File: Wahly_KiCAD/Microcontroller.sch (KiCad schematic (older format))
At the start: 21 parts, among them SW1 SW_SPDT, U5 STM32F302C8Tx, U6 W25Q32JVSS, Y1 16MHz

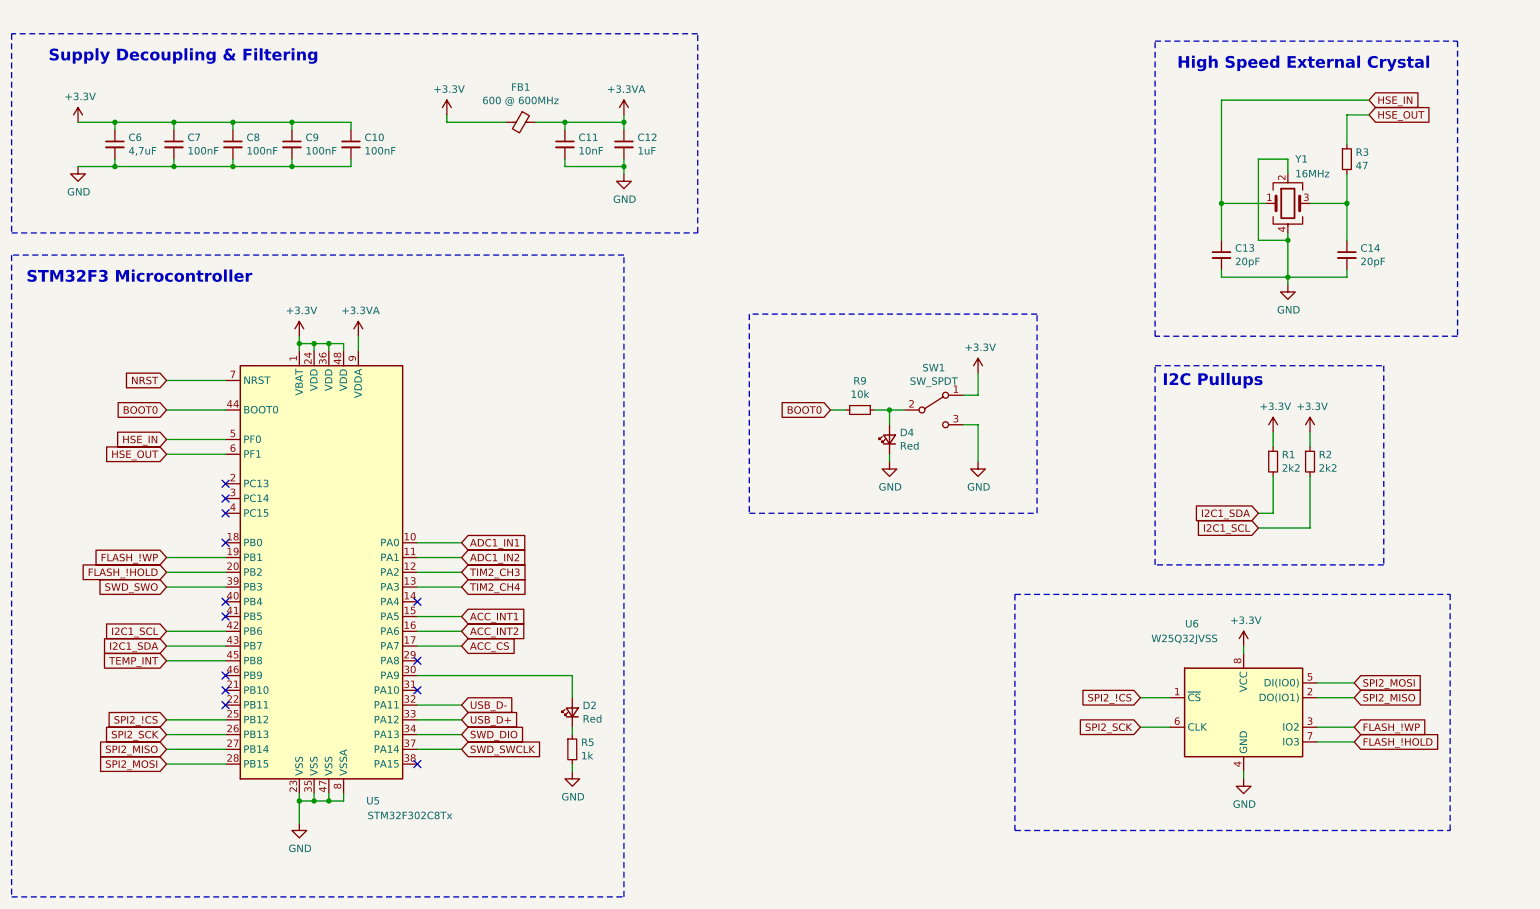
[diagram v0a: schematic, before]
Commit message: pdf schematic
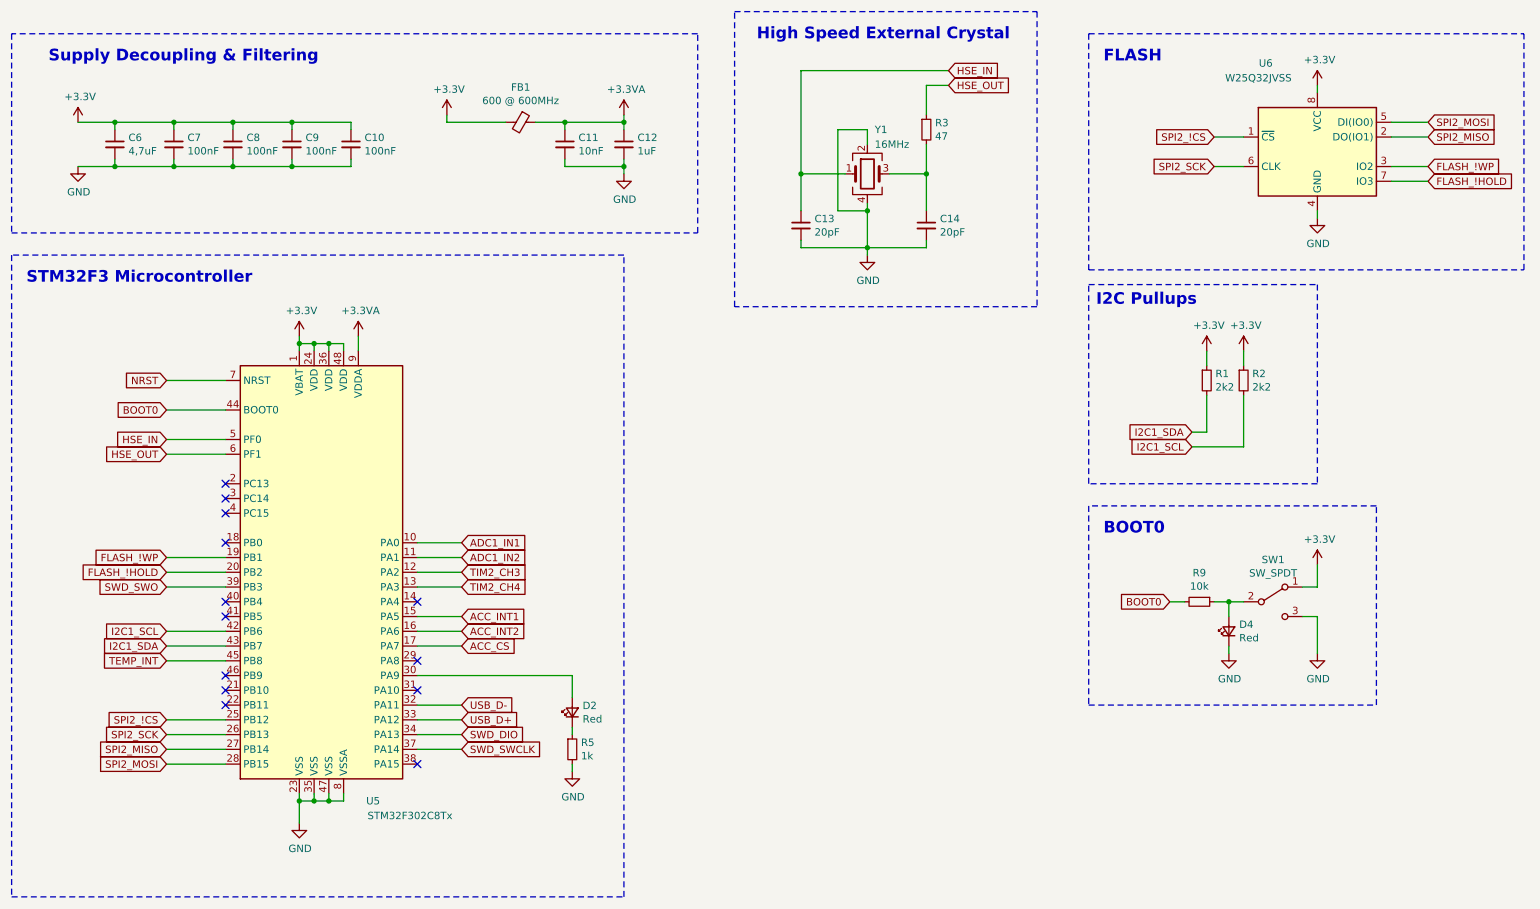
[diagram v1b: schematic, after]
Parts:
- R3: footprint Resistor_SMD:R_0603_1608Metric -> Resistor_SMD:R_0402_1005Metric
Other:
- note added: "BOOT0"
- note added: "FLASH"
- moved on the sheet: C13, C14, D4, R1, R2, R3, R9, SW1, U6, Y1
